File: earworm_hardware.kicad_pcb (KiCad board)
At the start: 4 copper layers, 19.1 x 26.3 mm, 40 parts, among them J1 Conn_01x05, J2 Conn_01x02, T1 LPR6235-752SMRC, U1 nRF54L15-QFXX, U2 ADXL367BCCZ-RL7, U3 LTC3108EDE-TRPBF, X1 32.768 kHz, X2 32MHz

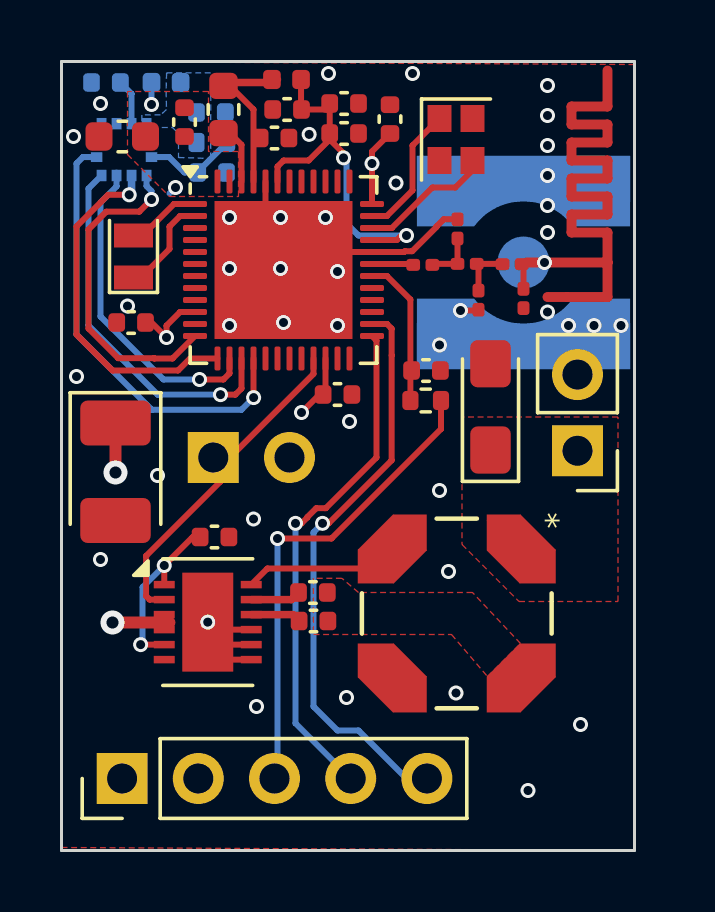
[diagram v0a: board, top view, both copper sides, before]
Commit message: changes from board review
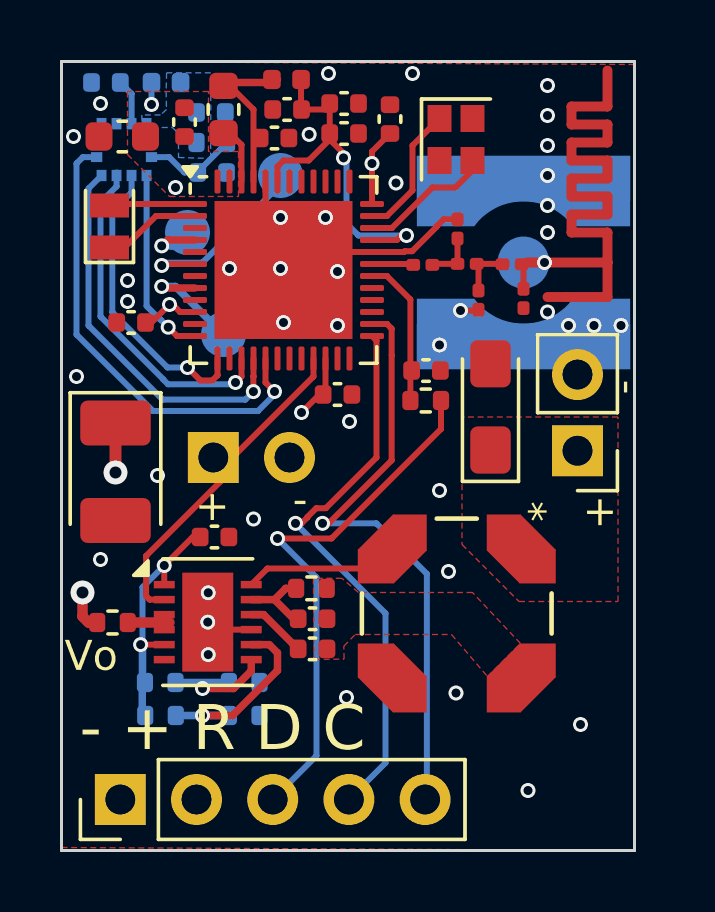
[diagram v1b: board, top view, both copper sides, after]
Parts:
- added R3: 500k, Resistor_SMD:R_0402_1005Metric, F.Cu at (99.9, 91.6)
- added R4: 0, Resistor_SMD:R_0402_1005Metric, F.Cu at (93.3, 92.7)
- added R5: 0, Resistor_SMD:R_0402_1005Metric, B.Cu at (97.7, 94.7)
- added R6: 0, Resistor_SMD:R_0402_1005Metric, B.Cu at (97.7, 95.8)
- added R7: 0, Resistor_SMD:R_0402_1005Metric, B.Cu at (94.9, 94.7)
- added R8: 0, Resistor_SMD:R_0402_1005Metric, B.Cu at (94.9, 95.8)
- added TP1: TestPoint, TestPoint:TestPoint_Pad_D1.5mm, B.Cu at (95.8, 79.7)
- added TP2: TestPoint, TestPoint:TestPoint_Pad_D1.5mm, B.Cu at (98.9, 77.8)
- added TP3: TestPoint, TestPoint:TestPoint_Pad_D1.5mm, B.Cu at (97.0, 83.1)
- moved X1 1.28 mm to (93.2, 79.5)
- moved C17 0.93 mm to (100.0, 93.6)
- moved C20 0.87 mm to (100.0, 92.6)
- moved J1 0.70 mm to (93.6, 98.6)
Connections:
- U1 pad 14: Net-(U1-P2.03) -> unconnected-(U1-P2.03-Pad14)
- U1 pad 17: unconnected-(U1-P2.06-Pad17) -> Net-(U1-P2.06)
- U1 pad 4: unconnected-(U1-P1.03-Pad4) -> Net-(U1-P1.03)
- U1 pad 6: unconnected-(U1-P1.05-Pad6) -> Net-(U1-P1.05)
- U1 pad 8: unconnected-(U1-P1.07-Pad8) -> Net-(U1-P1.07)
- U2 pad 3: Net-(U1-P2.03) -> Net-(U1-P2.04)
- U2 pad 4: Net-(U1-P2.04) -> Net-(U1-P2.05)
- U2 pad 5: Net-(U1-P2.05) -> Net-(U1-P2.06)
- U3 pad 3: VDD -> Net-(U3-VOUT)
- U3 pad 4: VDD -> Net-(U3-VOUT)
- U3 pad 7: GND -> Net-(U3-VS2)
- U3 pad 8: GND -> Net-(U3-VS1)
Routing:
- net Net-(U1-P2.06): track 0.00 -> 15.7 mm, vias 0 -> 1
- net Net-(U1-P2.03): track 10.8 -> 0.00 mm, vias 1 -> 0
- net Net-(U3-VS1): track 0.00 -> 6.57 mm, vias 0 -> 1
- net Net-(U1-P1.05): track 0.00 -> 6.21 mm, vias 0 -> 1
- net Net-(U1-P2.01): track 11.0 -> 6.38 mm
- net Net-(U3-VS2): track 0.00 -> 4.14 mm, vias 0 -> 1
- net Net-(U1-P1.07): track 0.00 -> 3.85 mm, vias 0 -> 1
- net Net-(U3-VAUX): track 5.98 -> 8.41 mm
- net Net-(U1-P1.03): track 0.00 -> 2.15 mm, vias 0 -> 1
- net Net-(U1-P2.05): track 14.9 -> 12.9 mm
- net Net-(U1-P2.02): track 11.8 -> 9.90 mm
- net /nRF54L15 RFSoC/NRST: track 16.0 -> 17.7 mm
- net /nRF54L15 RFSoC/SWDIO: track 17.0 -> 18.7 mm
- net GND: track 14.6 -> 13.1 mm
- net VDD: track 12.1 -> 10.7 mm
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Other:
- board text added: "+"
- board text added: "-"
- board text added: "- + R D C"
- board text added: "1+"
- board text added: "1-"
- board text added: "2+"
- board text added: "2-"
- board text added: "Vo"
